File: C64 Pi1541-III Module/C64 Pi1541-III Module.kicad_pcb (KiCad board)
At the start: 2 copper layers, 100 x 100 mm, 25 parts, among them J1 DC IN, J2 C64_IEC, J3 C64_IEC, J8 Module_Panel, M1 Mounting, M2 Mounting, M3 Mounting, M4 Mounting, U1 7406

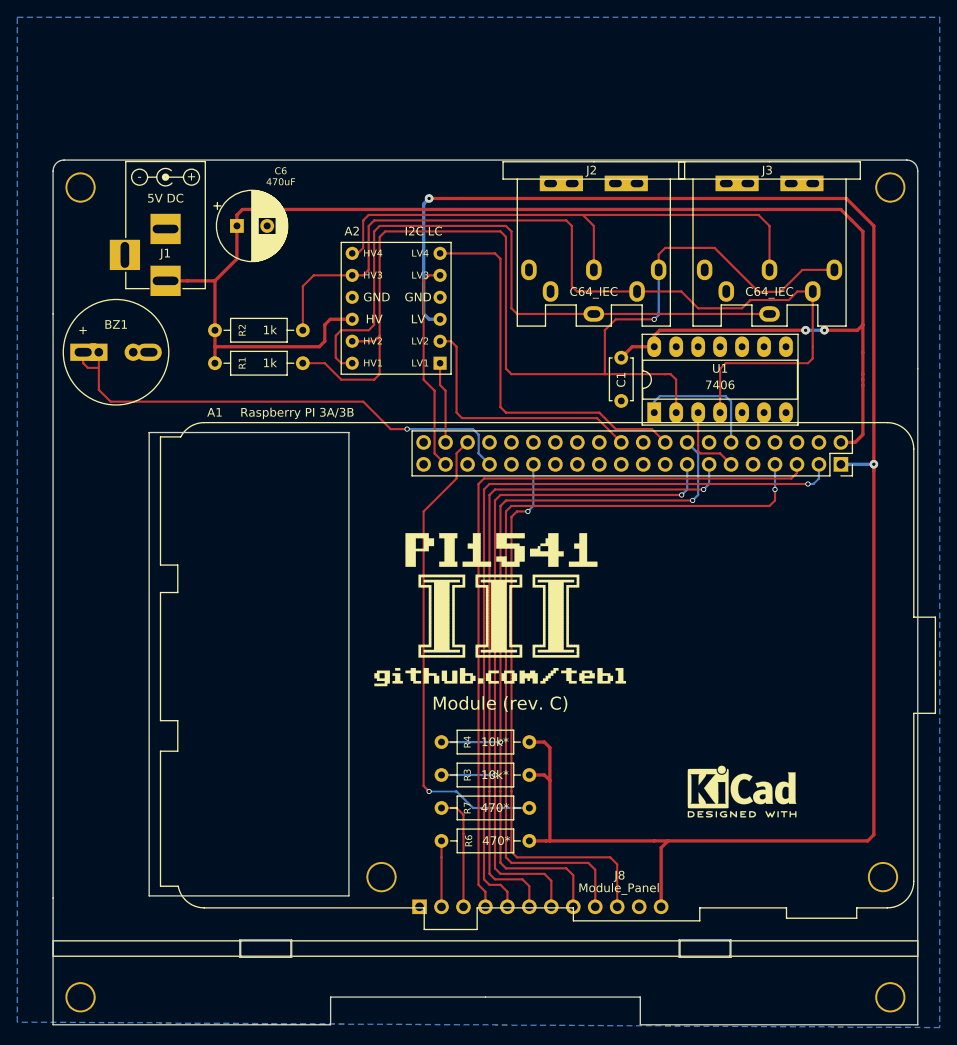
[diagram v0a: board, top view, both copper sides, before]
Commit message: ...
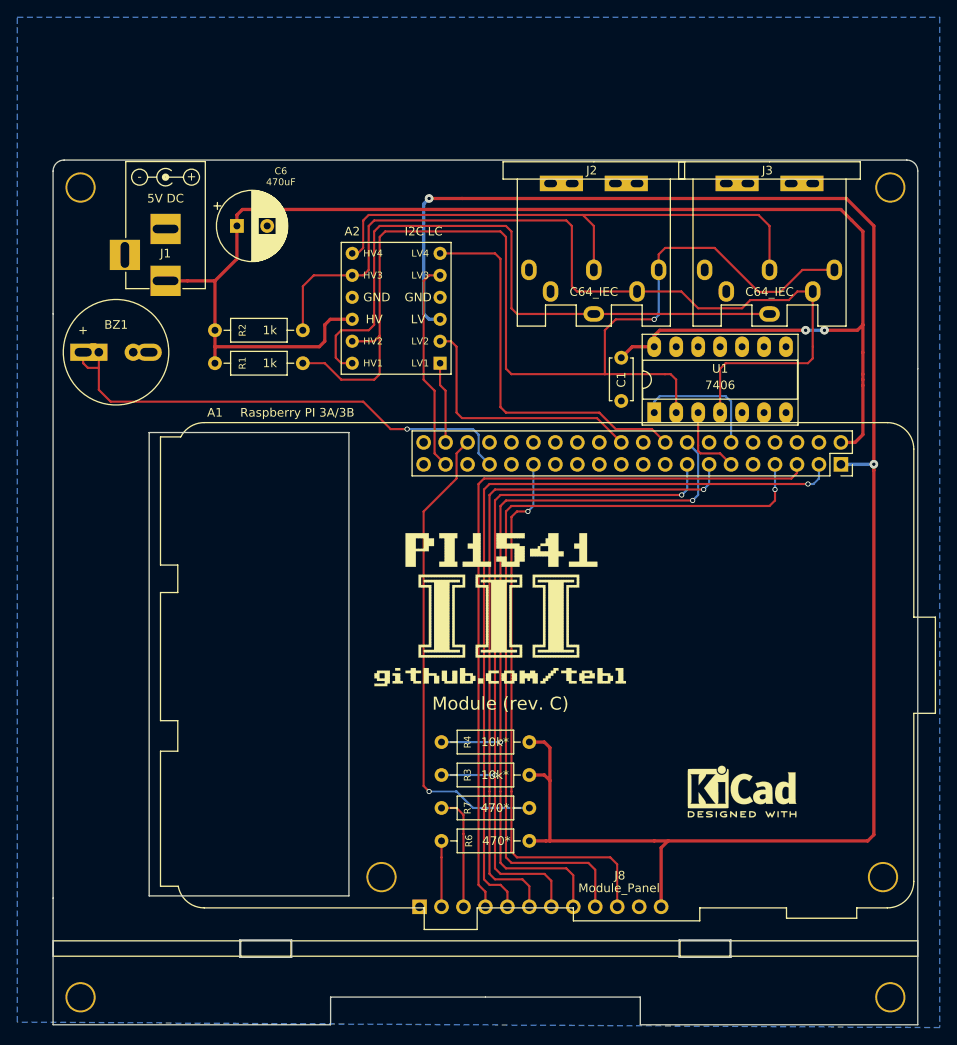
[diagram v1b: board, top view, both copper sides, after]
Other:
- net class Default removed
- net class Power removed
